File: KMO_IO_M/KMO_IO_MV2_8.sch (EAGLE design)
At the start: 106 parts, among them IC1 MCP23017SS, Q1 8MHz, Q2 25MHz, U1 ULN2803ADW

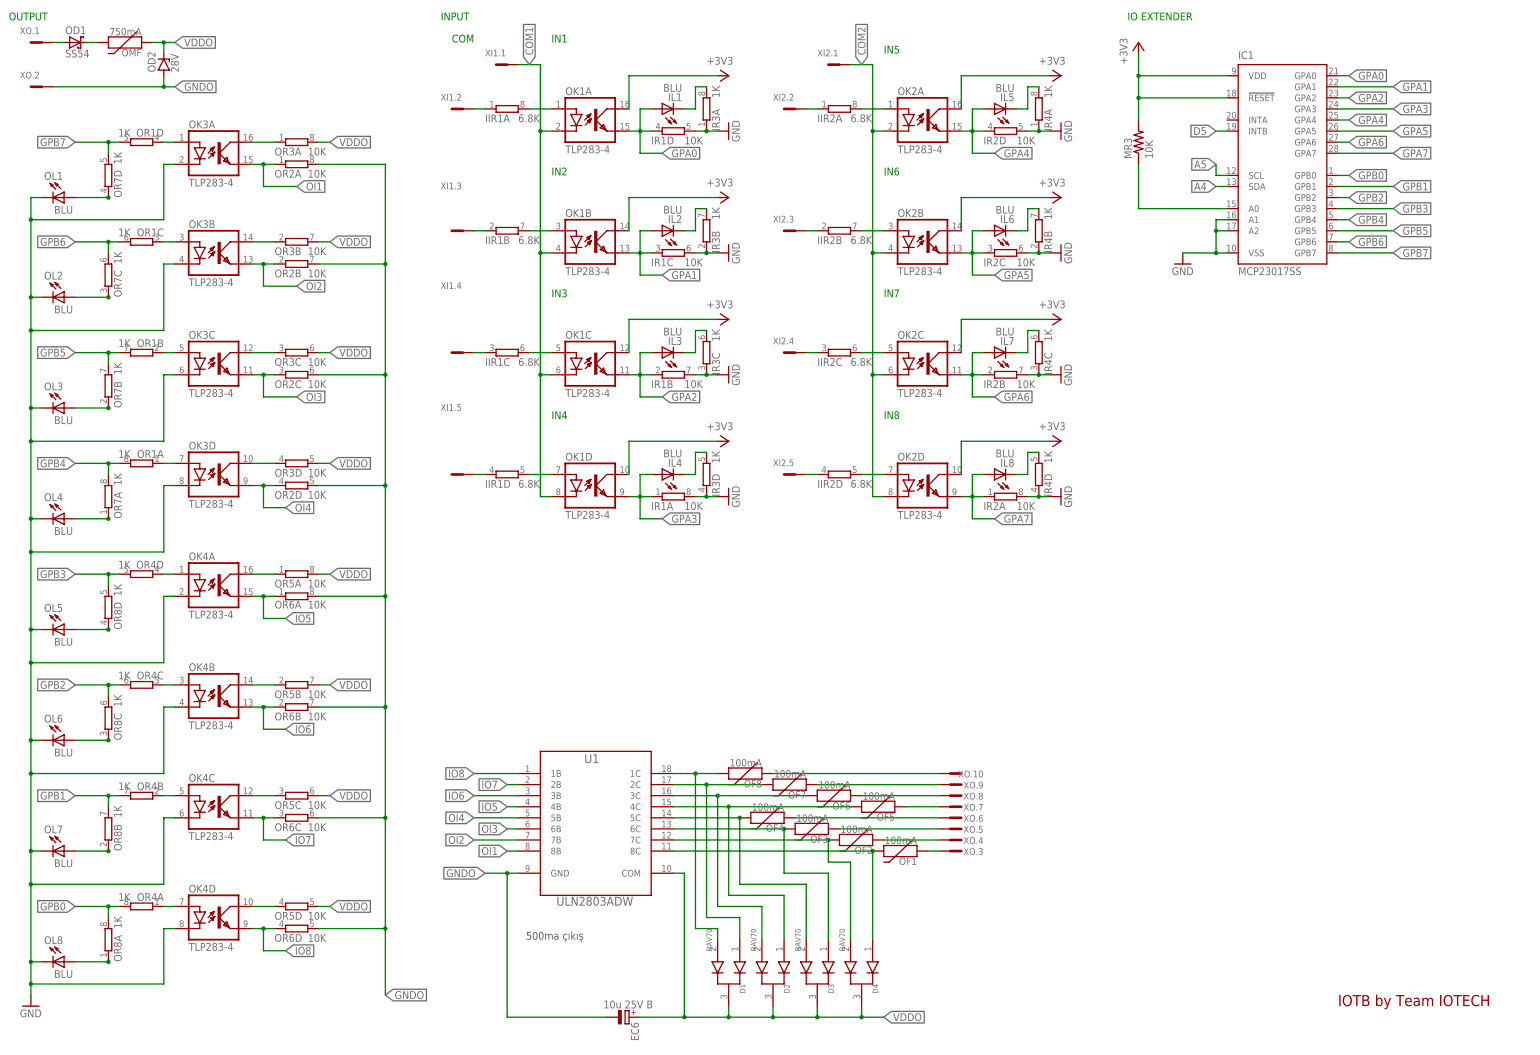
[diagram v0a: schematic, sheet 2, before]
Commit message: 2.8
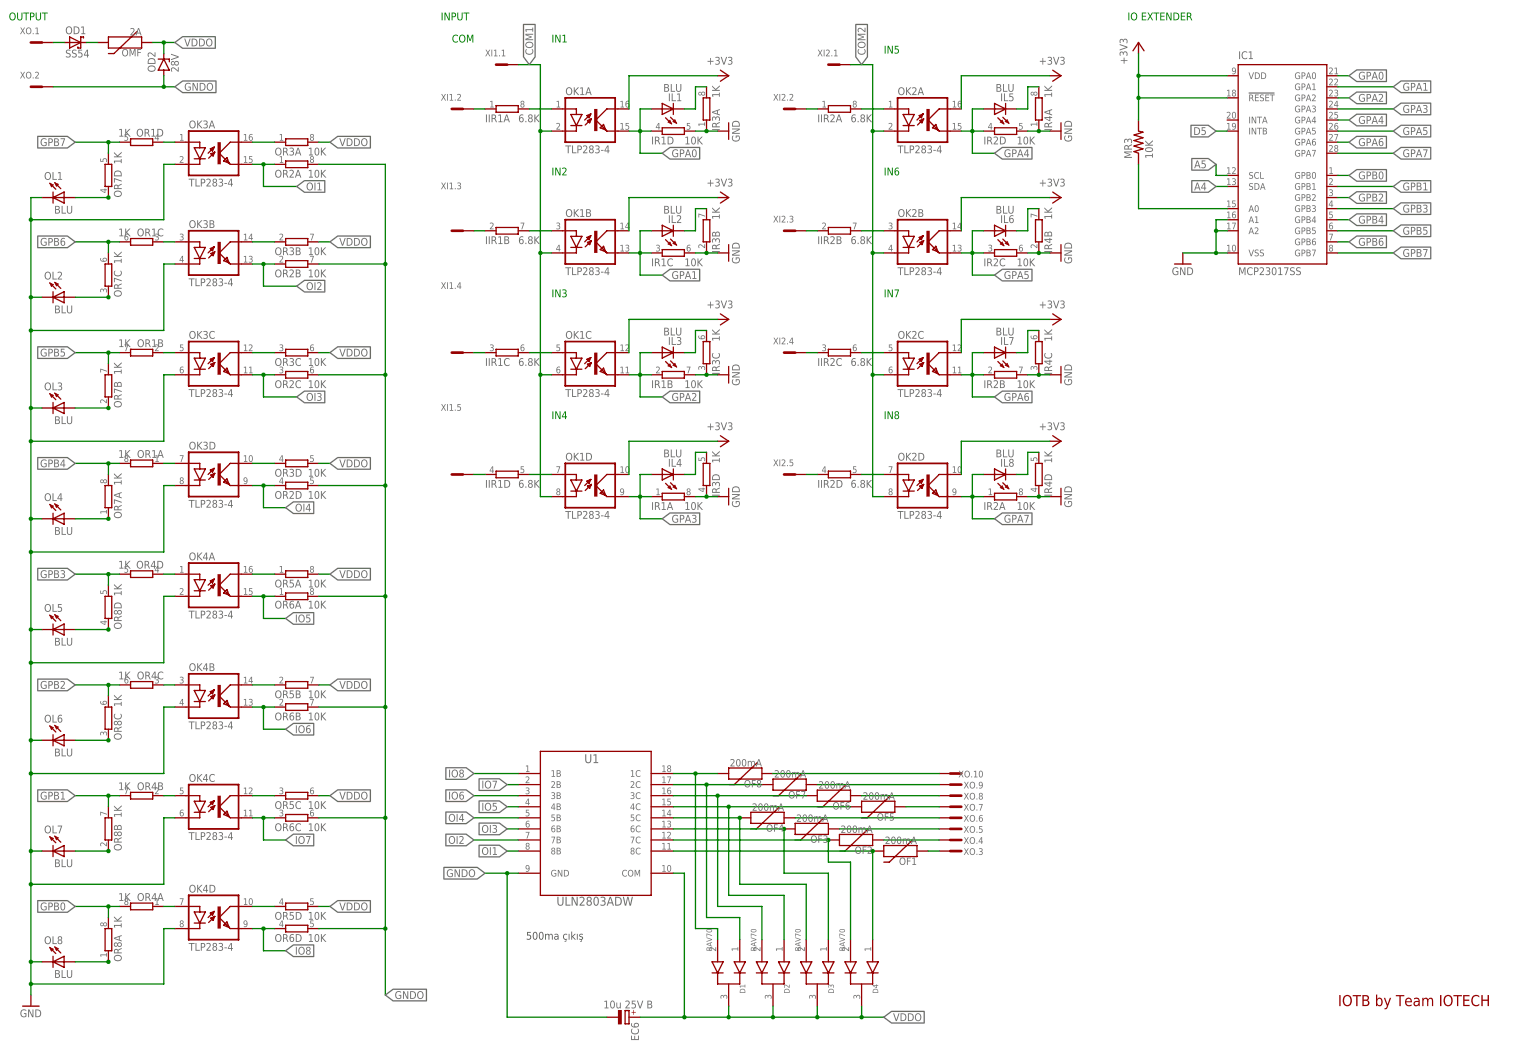
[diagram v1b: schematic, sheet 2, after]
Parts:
- OF1, OF2, OF3, OF4, OF5, OF6, OF7, OF8: value 100mA -> 200mA
- OMF: value 750mA -> 2A
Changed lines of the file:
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@@
 <part name="D3" library="BAV70" deviceset="BAV70" device="" override_package3d_urn="urn:adsk.eagle:package:10694704/2" override_package_urn="urn:adsk.eagle:footprint:10694705/1"/>
 <part name="D4" library="BAV70" deviceset="BAV70" device="" override_package3d_urn="urn:adsk.eagle:package:10694704/2" override_package_urn="urn:adsk.eagle:footprint:10694705/1"/>
-<part name="OF2" library="SparkFun-Fuses" deviceset="PPTC" device="_0.75A" override_package3d_urn="urn:adsk.eagle:package:10694727/2" override_package_urn="urn:adsk.eagle:footprint:10694728/1" value="100mA"/>
-<part name="OF3" library="SparkFun-Fuses" deviceset="PPTC" device="_0.75A" override_package3d_urn="urn:adsk.eagle:package:10694727/2" override_package_urn="urn:adsk.eagle:footprint:10694728/1" value="100mA"/>
-<part name="OF4" library="SparkFun-Fuses" deviceset="PPTC" device="_0.75A" override_package3d_urn="urn:adsk.eagle:package:10694727/2" override_package_urn="urn:adsk.eagle:footprint:10694728/1" value="100mA"/>
-<part name="OF5" library="SparkFun-Fuses" deviceset="PPTC" device="_0.75A" override_package3d_urn="urn:adsk.eagle:package:10694727/2" override_package_urn="urn:adsk.eagle:footprint:10694728/1" value="100mA"/>
-<part name="OF6" library="SparkFun-Fuses" deviceset="PPTC" device="_0.75A" override_package3d_urn="urn:adsk.eagle:package:10694727/2" override_package_urn="urn:adsk.eagle:footprint:10694728/1" value="100mA"/>
-<part name="OF7" library="SparkFun-Fuses" deviceset="PPTC" device="_0.75A" override_package3d_urn="urn:adsk.eagle:package:10694727/2" override_package_urn="urn:adsk.eagle:footprint:10694728/1" value="100mA"/>
-<part name="OF8" library="SparkFun-Fuses" deviceset="PPTC" device="_0.75A" override_package3d_urn="urn:adsk.eagle:package:10694727/2" override_package_urn="urn:adsk.eagle:footprint:10694728/1" value="100mA"/>
-<part name="OMF" library="SparkFun-Fuses" deviceset="PPTC" device="_0.75A" override_package3d_urn="urn:adsk.eagle:package:10694727/2" override_package_urn="urn:adsk.eagle:footprint:10694728/1" value="750mA"/>
-<part name="OF1" library="SparkFun-Fuses" deviceset="PPTC" device="_0.75A" override_package3d_urn="urn:adsk.eagle:package:10694727/2" override_package_urn="urn:adsk.eagle:footprint:10694728/1" value="100mA"/>
+<part name="OF2" library="SparkFun-Fuses" deviceset="PPTC" device="_0.75A" override_package3d_urn="urn:adsk.eagle:package:10694727/2" override_package_urn="urn:adsk.eagle:footprint:10694728/1" value="200mA"/>
+<part name="OF3" library="SparkFun-Fuses" deviceset="PPTC" device="_0.75A" override_package3d_urn="urn:adsk.eagle:package:10694727/2" override_package_urn="urn:adsk.eagle:footprint:10694728/1" value="200mA"/>
+<part name="OF4" library="SparkFun-Fuses" deviceset="PPTC" device="_0.75A" override_package3d_urn="urn:adsk.eagle:package:10694727/2" override_package_urn="urn:adsk.eagle:footprint:10694728/1" value="200mA"/>
+<part name="OF5" library="SparkFun-Fuses" deviceset="PPTC" device="_0.75A" override_package3d_urn="urn:adsk.eagle:package:10694727/2" override_package_urn="urn:adsk.eagle:footprint:10694728/1" value="200mA"/>
+<part name="OF6" library="SparkFun-Fuses" deviceset="PPTC" device="_0.75A" override_package3d_urn="urn:adsk.eagle:package:10694727/2" override_package_urn="urn:adsk.eagle:footprint:10694728/1" value="200mA"/>
+<part name="OF7" library="SparkFun-Fuses" deviceset="PPTC" device="_0.75A" override_package3d_urn="urn:adsk.eagle:package:10694727/2" override_package_urn="urn:adsk.eagle:footprint:10694728/1" value="200mA"/>
+<part name="OF8" library="SparkFun-Fuses" deviceset="PPTC" device="_0.75A" override_package3d_urn="urn:adsk.eagle:package:10694727/2" override_package_urn="urn:adsk.eagle:footprint:10694728/1" value="200mA"/>
+<part name="OMF" library="SparkFun-Fuses" deviceset="PPTC" device="_0.75A" override_package3d_urn="urn:adsk.eagle:package:10694727/2" override_package_urn="urn:adsk.eagle:footprint:10694728/1" value="2A"/>
+<part name="OF1" library="SparkFun-Fuses" deviceset="PPTC" device="_0.75A" override_package3d_urn="urn:adsk.eagle:package:10694727/2" override_package_urn="urn:adsk.eagle:footprint:10694728/1" value="200mA"/>
 <part name="IR3" library="resistor-dil" library_urn="urn:adsk.eagle:library:342" deviceset="4R-N" device="0603-ARV" package3d_urn="urn:adsk.eagle:package:24915/1" override_package3d_urn="urn:adsk.eagle:package:10705410/2" override_package_urn="urn:adsk.eagle:footprint:24895/1" value="1K"/>
 <part name="IR4" library="resistor-dil" library_urn="urn:adsk.eagle:library:342" deviceset="4R-N" device="0603-ARV" package3d_urn="urn:adsk.eagle:package:24915/1" override_package3d_urn="urn:adsk.eagle:package:10705410/2" override_package_urn="urn:adsk.eagle:footprint:24895/1" value="1K"/>
